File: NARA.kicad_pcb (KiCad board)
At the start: 4 copper layers, 93.9 x 42.4 mm, 140 parts, among them K1 BATT, K10 TOF_LD, K11 TOF_LS, K12 TOF_RF, K13 TOF_RD, K14 TOF_RS, K2 K_FPC_52435-2471, K3 PROG, K5 K_PicoSPOX-3, K6 K_0002, K7 K_PicoSPOX-3, K8 K_0002, K9 TOF_LF, Q1 Q_0004, Q2 Q_0007, Q3 Q_0007, Q4 Q_0007, Q5 Q_0007, Q6 Q_0007, Q7 Q_0007, Q8 Q_0004, Q9 Q_0004, SW1 SW_SKQG, SW2 SW_SKQG, U1 U_LT8610ABIMSE-3.3, U10 QRE1113GR, U11 QRE1113GR, U12 QRE1113GR, U2 U_AP2204K-5.0TRG1, U3 LTC2944, U4 L6234, U5 L6234, U6 LTC2955TS8-1, U7 STM32H743VITx, U8 ICM-20689, U9 QRE1113GR

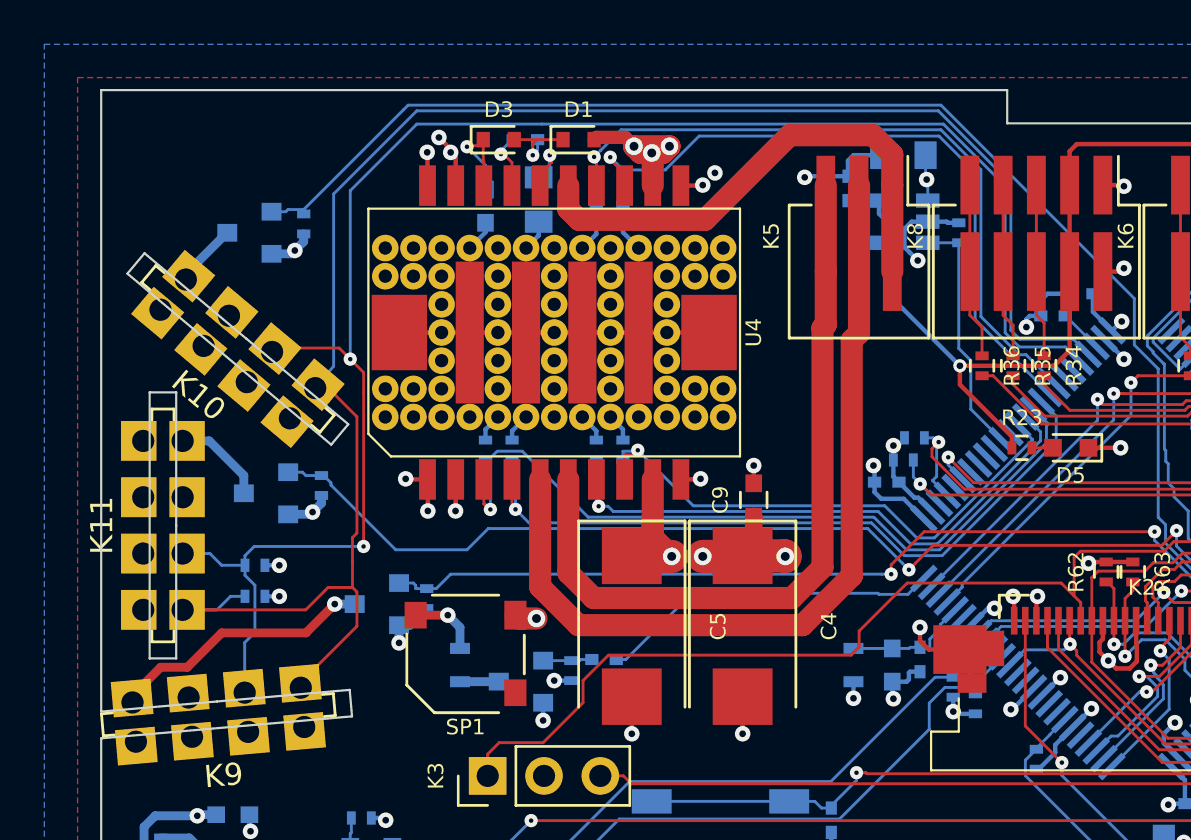
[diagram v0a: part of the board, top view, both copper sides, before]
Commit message: Save before change vias
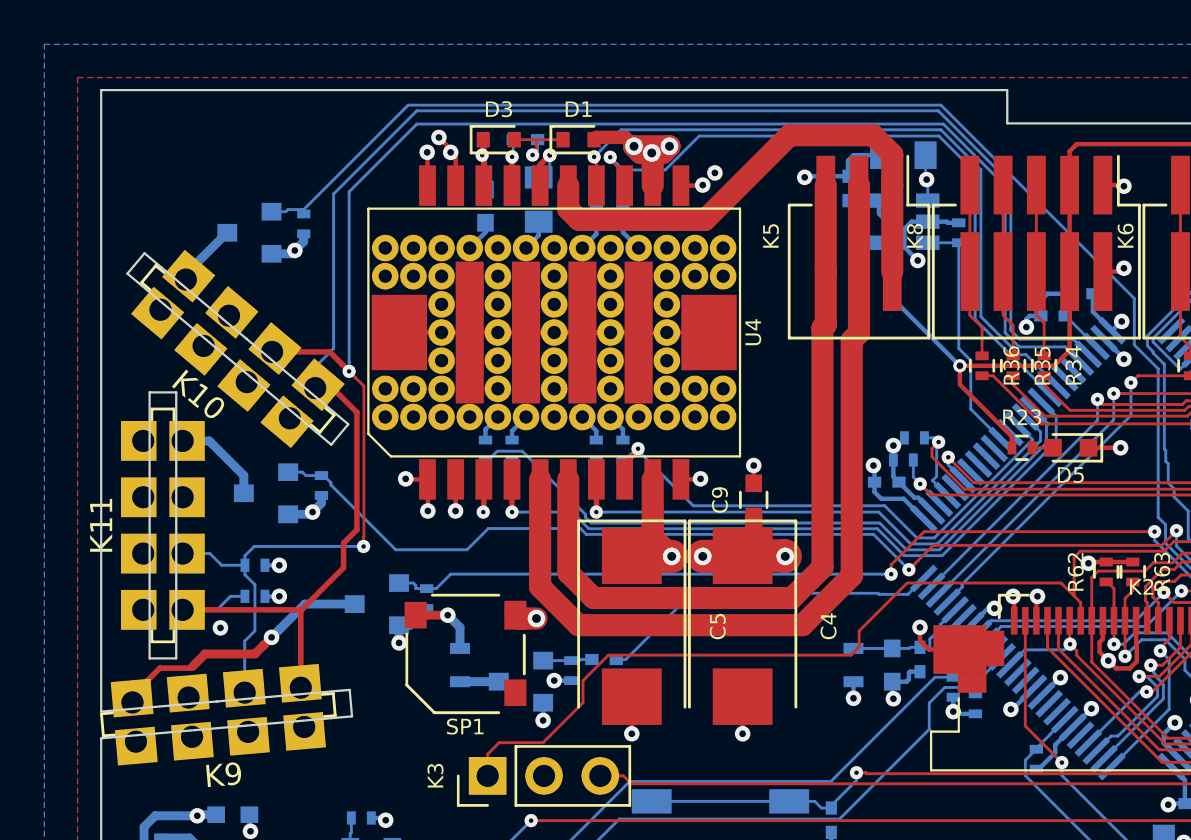
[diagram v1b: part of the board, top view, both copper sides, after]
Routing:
- net /TOF_L_SDA: track 80.1 -> 78.2 mm
- net Net-(C18-Pad1): track 5.12 -> 4.42 mm
- net Net-(C12-Pad1): track 2.61 -> 2.10 mm
- net GND: track 801.5 -> 801.6 mm, vias 87 -> 88
- net Net-(C15-Pad2): track 3.45 -> 3.39 mm, vias 1 -> 2
